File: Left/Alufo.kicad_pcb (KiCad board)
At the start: 2 copper layers, 139.7 x 88.9 mm, 67 parts, among them J1 USB_C_Receptacle_USB2.0_16P_2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, J3 USB_C_Receptacle_USB2.0_16P_2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, K11 PG1350, K12 PG1350, K13 PG1350, K14 PG1350, K15 PG1350, K16 PG1350, K21 PG1350, K22 PG1350, K23 PG1350, K24 PG1350, K25 PG1350, K26 PG1350, K31 PG1350, K32 PG1350, K33 PG1350, K34 PG1350, K35 PG1350, K36 PG1350_1½U, SW1 BOOT, U1 CH552T, U3 USBLC6-2P6, U5 USBLC6-2P6

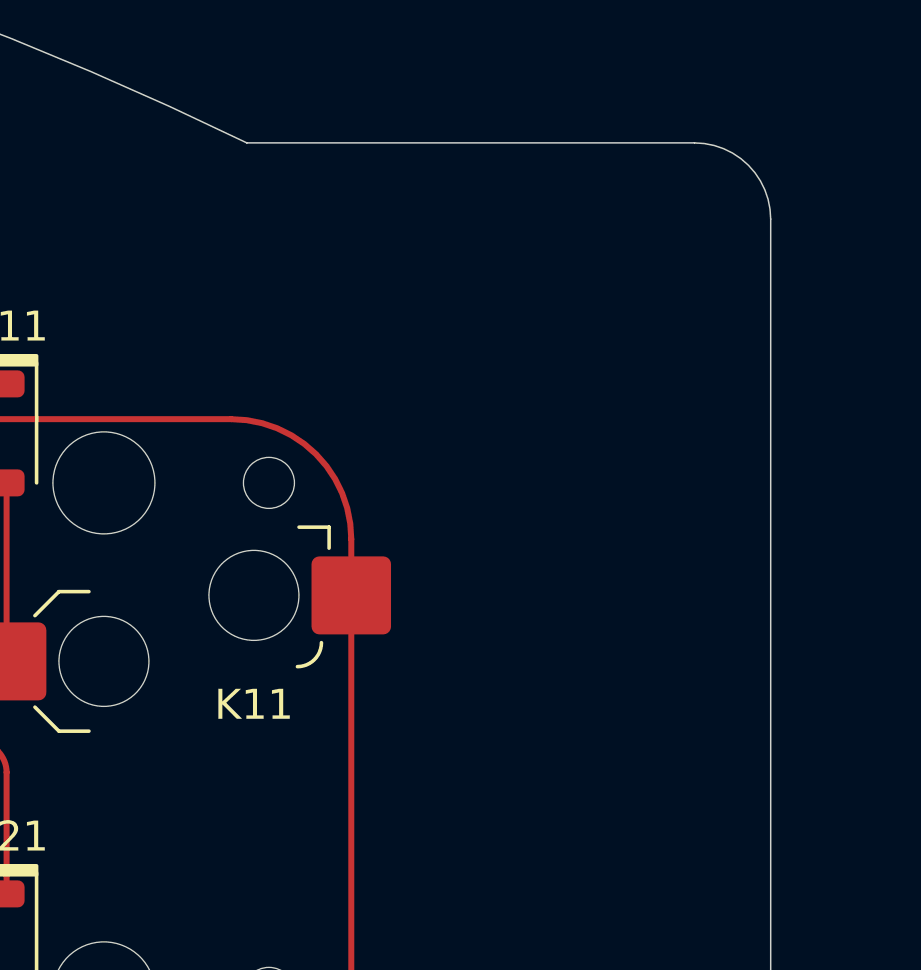
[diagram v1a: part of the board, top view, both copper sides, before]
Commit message: Add fun logo on lefthand board
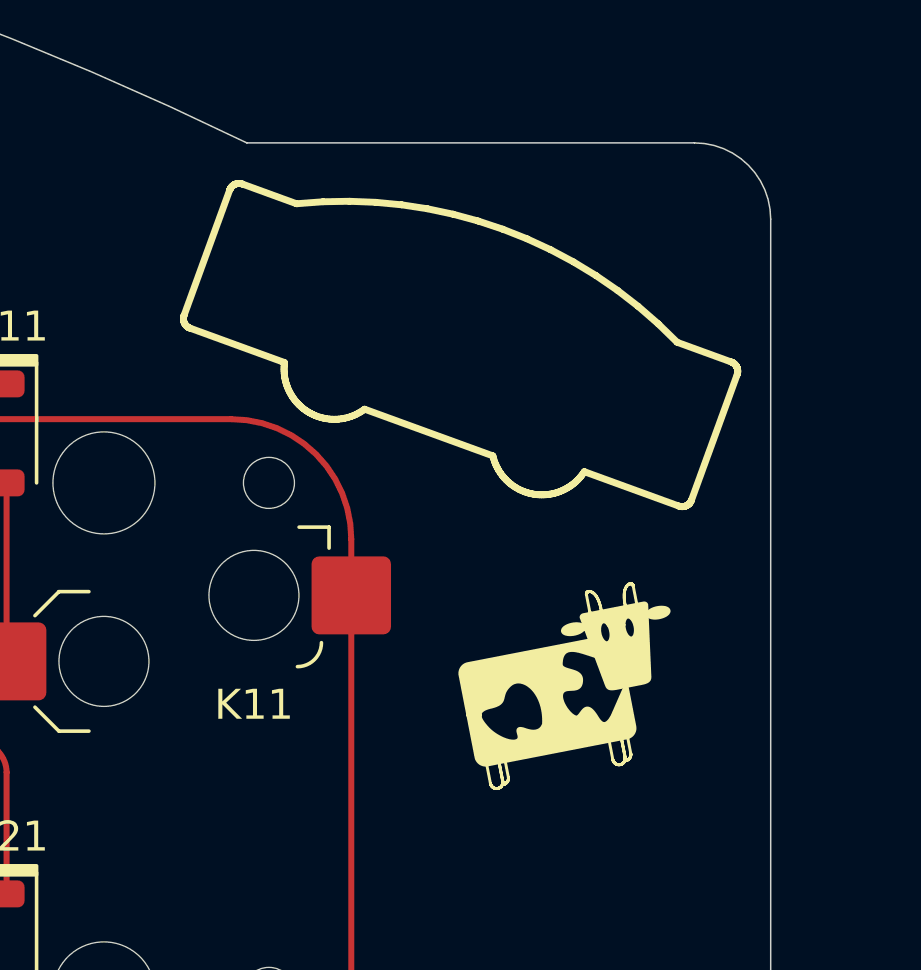
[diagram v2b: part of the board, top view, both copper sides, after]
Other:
- board text added: "${PROJECTNAME} v${PCB_REVISION} • ${AUTHOR}"
- board text removed: "${AUTHOR}"
